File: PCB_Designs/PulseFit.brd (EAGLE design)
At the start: 50.8 x 56.1 mm, 54 parts

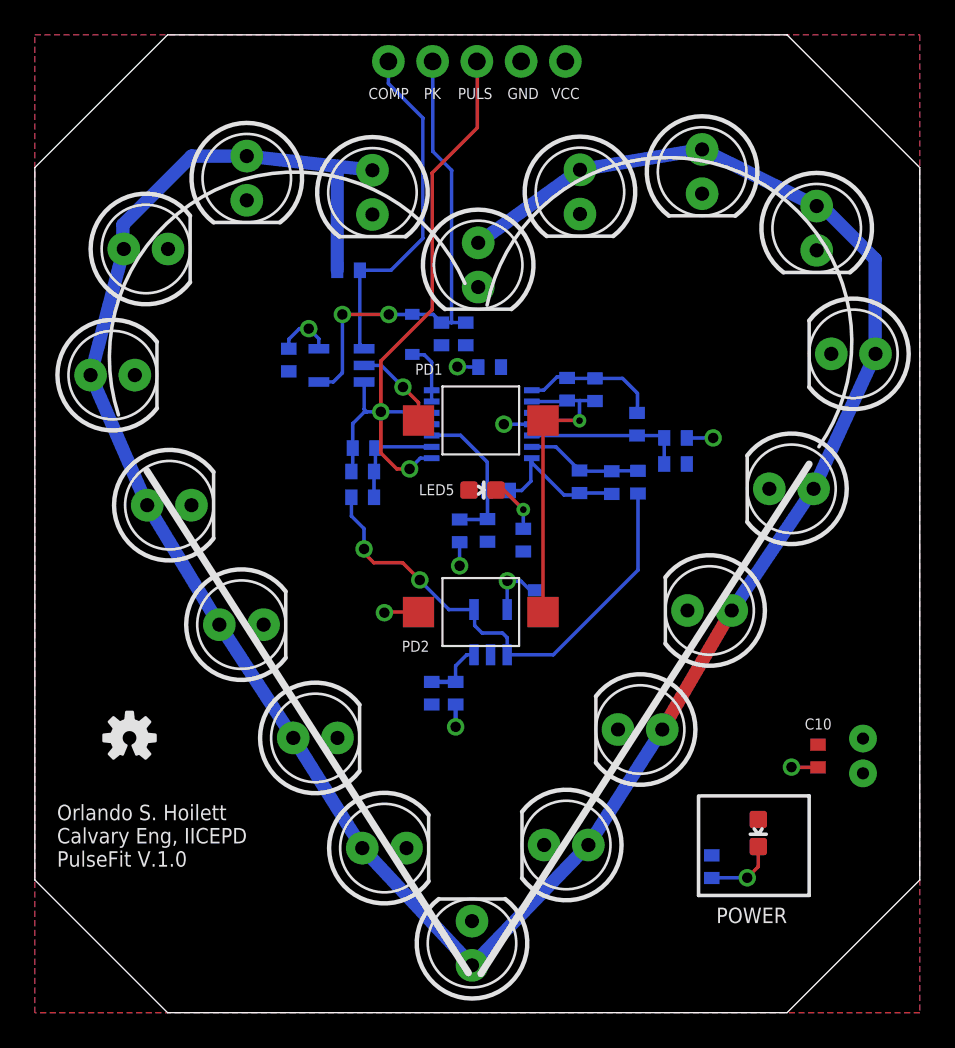
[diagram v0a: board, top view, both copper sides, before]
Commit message: updates
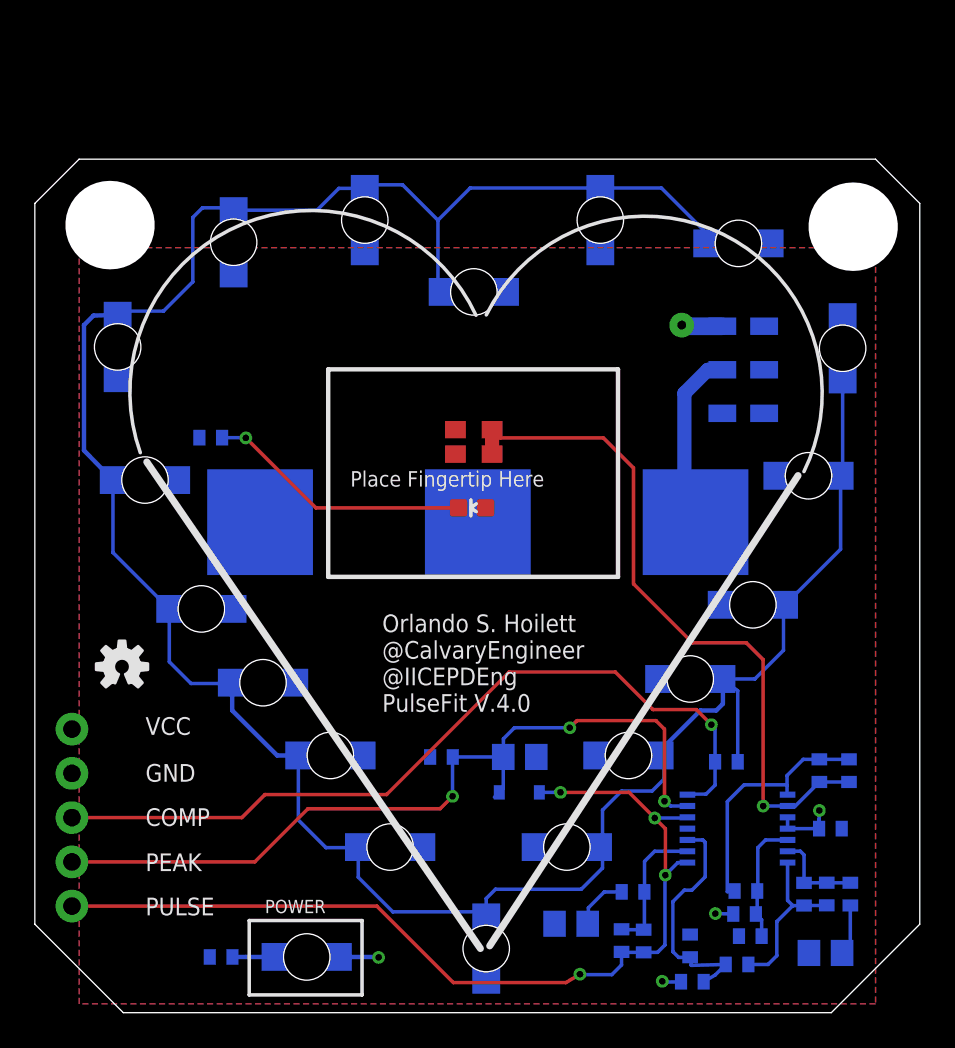
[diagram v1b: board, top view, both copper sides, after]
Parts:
- removed C10, C9: 100n, resistor:C0402
- removed COMP, VREF: AD8603UJ, analog-devices:SOT23-5
- removed JST: JST-PTH, Orlando:JST-2-PTH-VERT
- removed LED1, LED10, LED12, LED16, LED2, LED22, LED23, LED24, LED25, LED26, LED28, LED3, LED4, LED6, LED7, LED8, LED9: (no value), SparkFun-LED:LED5MM
- removed LED5: (no value), SparkFun-LED:LED-0603
- removed PD1, PD2: PD-ODD-900-001, Orlando:SMD-PD-01
- removed R6, R7: 49.9k, resistor:R0402
- added BATT-CR2032: (no value), SparkFun-Electromechanical:BATTCON_20MM
- added C11: 10n, resistor:C0402
- added LD1, LD10, LD12, LD13, LD14, LD15, LD16, LD17, LD18, LD2, LD3, LD4, LD5, LD6, LD7, LD8, LD9, LED13: LED-LTST-C230KRKT, Orlando:LED-1206-BOTTOM
- added PD: LED-PD15-22B_TR8, Orlando:LED-PD15-22B_TR8
- added PULSE: (no value), SparkFun-LED:LED-0603
- C1: value 33n -> 1uF
- C2, C4: value 570n -> 1u
- C3: value 318n -> 10u; device resistor:C0402 -> resistor:C0805
- C5: value 318n -> 10n
- C6: device resistor:C0402 -> resistor:C0805
- C7: value 100n -> 10n
- C8: value 100n -> 10u; device resistor:C0402 -> resistor:C0805
- GAIN: value AD8609RU -> MCP6004
- LED11: value (none) -> LED-LTST-C230KRKT; device SparkFun-LED:LED5MM -> Orlando:LED-1206-BOTTOM
- POWER: value ON -> SWITCH-DPDT-JS202011JCQN; device SparkFun-LED:LED-0603 -> SparkFun-Electromechanical:J-LEAD
- R1: value 1M -> 32k
- R10: value 100k -> 3.3M
- R11, R5: value 10k -> 32k
- R13: value (none) -> 169
- R14: value 100 -> 1k
- R2: value 1M -> 3.3M
- R3, R8, R9: value 1M -> 1.5M
- R4: value 100k -> 1.5M
- moved BREAKOUT 51.8 mm to (27.5, 6.12), turned to 90 degrees
- moved C8 45.9 mm to (70.8, 3.43), turned to 180 degrees
- moved R13 35.6 mm to (65.1, 14.4), turned to 180 degrees
- moved C7 32.9 mm to (71.1, 10.6)
- moved C5 31.9 mm to (59.1, 4.14), turned to 270 degrees
- moved R10 31.4 mm to (60.4, 4.11), turned to 270 degrees
- moved C4 30.5 mm to (65.7, 2.77)
- moved R8 29.1 mm to (63.1, 1.78), turned to 180 degrees
- moved R15 28.6 mm to (36.1, 3.20), turned to 0 degrees
- moved R4 27.9 mm to (66.5, 4.39), turned to 0 degrees
- moved C2 27.5 mm to (66.2, 6.99), turned to 180 degrees
- moved GAIN 27.5 mm to (65.7, 10.6)
- moved R11 27.5 mm to (59.7, 6.93)
- moved R2 27.2 mm to (69.6, 6.80), turned to 270 degrees
- moved D1 27.0 mm to (53.2, 12.6), turned to 180 degrees
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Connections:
- removed net 1/2-VDD: R11.1, R5.1, VREF.1, VREF.4
- removed net N$7: R6.1, R7.2, VREF.3
- new net N$11: C11.2, C4.1, GAIN.7, R2.2
- new net N$14: C8.2, R5.1
- net ANODE: now also LD1.A, LD10.A, LD12.A, LD13.A, LD14.A, LD15.A, LD16.A, LD17.A, LD18.A, LD2.A, LD3.A, LD4.A, LD5.A, LD6.A, LD7.A, LD8.A, LD9.A; no longer LED1.A, LED10.A, LED12.A, LED16.A, LED2.A, LED22.A, LED23.A, LED24.A, LED25.A, LED26.A, LED28.A, LED3.A, LED4.A, LED6.A, LED7.A, LED8.A, LED9.A
- net COMP: now also BREAKOUT.3, GAIN.14; no longer BREAKOUT.1, COMP.1
- net GND: now also BATT-CR2032.2, C3.1, C8.1, LD1.C, LD10.C, LD12.C, LD13.C, LD14.C, LD15.C, LD16.C, LD17.C, LD18.C, LD2.C, LD3.C, LD4.C, LD5.C, LD6.C, LD7.C, LD8.C, LD9.C, LED11.C, POWER.4, POWER.5, POWER.6, R4.2; no longer C10.2, C8.2, C9.2, COMP.2, GAIN.3, JST.-, LED1.K, LED10.K, LED11.K, LED12.K, LED16.K, LED2.K, LED22.K, LED23.K, LED24.K, LED25.K, LED26.K, LED28.K, LED3.K, LED4.K, LED6.K, LED7.K, LED8.K, LED9.K, PD1.ANODE, PD2.ANODE, R3.2, R6.2, VREF.2
- net N$1: now also PD.A-1, PD.A-2; no longer PD1.CATHODE, PD2.CATHODE
- net N$10: now also C11.1, GAIN.6, R2.1, R5.2; no longer D1.A, GAIN.13, GAIN.14
- net N$12: now also LED13.C; no longer POWER.C
- net N$4: now also R3.2, R4.1; no longer R2.2, R3.1
- net N$5: now also BATT-CR2032.1, POWER.2; no longer C3.1, GAIN.6, R4.1, R5.2
- net N$6: now also R11.1; no longer C4.1, GAIN.7, R4.2
- net N$9: now also PULSE.C; no longer LED5.C
- net PEAK: now also GAIN.13; no longer COMP.4
- net PULSE: now also BREAKOUT.1, D1.A; no longer BREAKOUT.3, COMP.3
- net VCC: now also GAIN.3, LED13.A, PD.C-1, PD.C-2, POWER.1, PULSE.A, R3.1; no longer C10.1, C8.1, C9.1, COMP.5, JST.+, LED5.A, POWER.A, R2.1, R7.1, VREF.5
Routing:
- net 1/2-VDD: track 29.2 -> 0.00 mm, vias 2 -> 0
- net COMP: track 20.0 -> 46.8 mm, vias 0 -> 1
- net N$1: track 17.9 -> 40.5 mm
- net PEAK: track 27.7 -> 47.6 mm, vias 2 -> 3
- net PULSE: track 38.2 -> 55.4 mm, vias 2 -> 4
- net N$9: track 3.13 -> 15.2 mm
- net N$11: track 0.00 -> 9.65 mm
- net GND: track 8.54 -> 0.00 mm, vias 3 -> 0
- net N$2: track 7.91 -> 14.5 mm
- net N$6: track 8.47 -> 3.23 mm
- net N$3: track 8.73 -> 13.6 mm
- net ANODE: track 145.5 -> 150.0 mm
- net N$5: track 6.68 -> 10.4 mm
- net N$7: track 3.61 -> 0.00 mm
- net VCC: track 13.8 -> 10.3 mm, vias 7 -> 5
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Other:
- board size 50.8 x 56.1 mm -> 50.8 x 49 mm
- board text added: "Creative Commons License Attribution-NonCommercial- ShareAlike 3.0 Unported"
- board text added: "Orlando S. Hoilett @CalvaryEngineer @IICEPDEng PulseFit V.4.0"
- board text added: "PEAK"
- board text added: "POWER"
- board text added: "PULSE"
- board text added: "Place Fingertip Here"
- board text removed: "Orlando S. Hoilett Calvary Eng, IICEPD PulseFit V.1.0"
- board text removed: "PK"
- board text removed: "PULS"

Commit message: updated PulseFit BOM and added disclaimer in schematic
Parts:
- C1: value 1uF -> 470n
- C2, C4: value 1u -> 470n
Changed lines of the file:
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@@
 <?xml version="1.0" encoding="utf-8"?>
 <!DOCTYPE eagle SYSTEM "eagle.dtd">
-<eagle version="7.4.0">
+<eagle version="7.3.0">
 <drawing>
 <settings>
@@
 </autorouter>
 <elements>
-<element name="C1" library="resistor" package="C0402" value="1uF" x="72.136" y="13.8938" smashed="yes" rot="MR90">
+<element name="C1" library="resistor" package="C0402" value="470n" x="72.136" y="13.8938" smashed="yes" rot="MR90">
 <attribute name="NAME" x="72.7202" y="15.2908" size="0.762" layer="26" rot="MR0"/>
 <attribute name="VALUE" x="70.231" y="13.2588" size="1.27" layer="28" rot="MR90"/>
 </element>
-<element name="C4" library="resistor" package="C0402" value="1u" x="65.7098" y="2.7686" smashed="yes" rot="MR0">
+<element name="C4" library="resistor" package="C0402" value="470n" x="65.7098" y="2.7686" smashed="yes" rot="MR0">
 <attribute name="NAME" x="67.8942" y="2.5654" size="0.762" layer="26" rot="MR270"/>
 <attribute name="VALUE" x="66.3448" y="0.8636" size="1.27" layer="28" rot="MR0"/>
@@
 <attribute name="VALUE" x="54.9148" y="7.6454" size="1.27" layer="28" rot="MR180"/>
 </element>
-<element name="C2" library="resistor" package="C0402" value="1u" x="66.2178" y="6.985" smashed="yes" rot="MR180">
+<element name="C2" library="resistor" package="C0402" value="470n" x="66.2178" y="6.985" smashed="yes" rot="MR180">
 <attribute name="NAME" x="64.1096" y="6.4008" size="0.762" layer="26" rot="MR90"/>
 <attribute name="VALUE" x="65.5828" y="8.89" size="1.27" layer="28" rot="MR180"/>
